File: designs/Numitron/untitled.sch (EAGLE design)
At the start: 10 parts, among them IC2 TLC5916IN, IC3 TLC5916IN, IC4 TLC5916IN, IC5 TLC5916IN

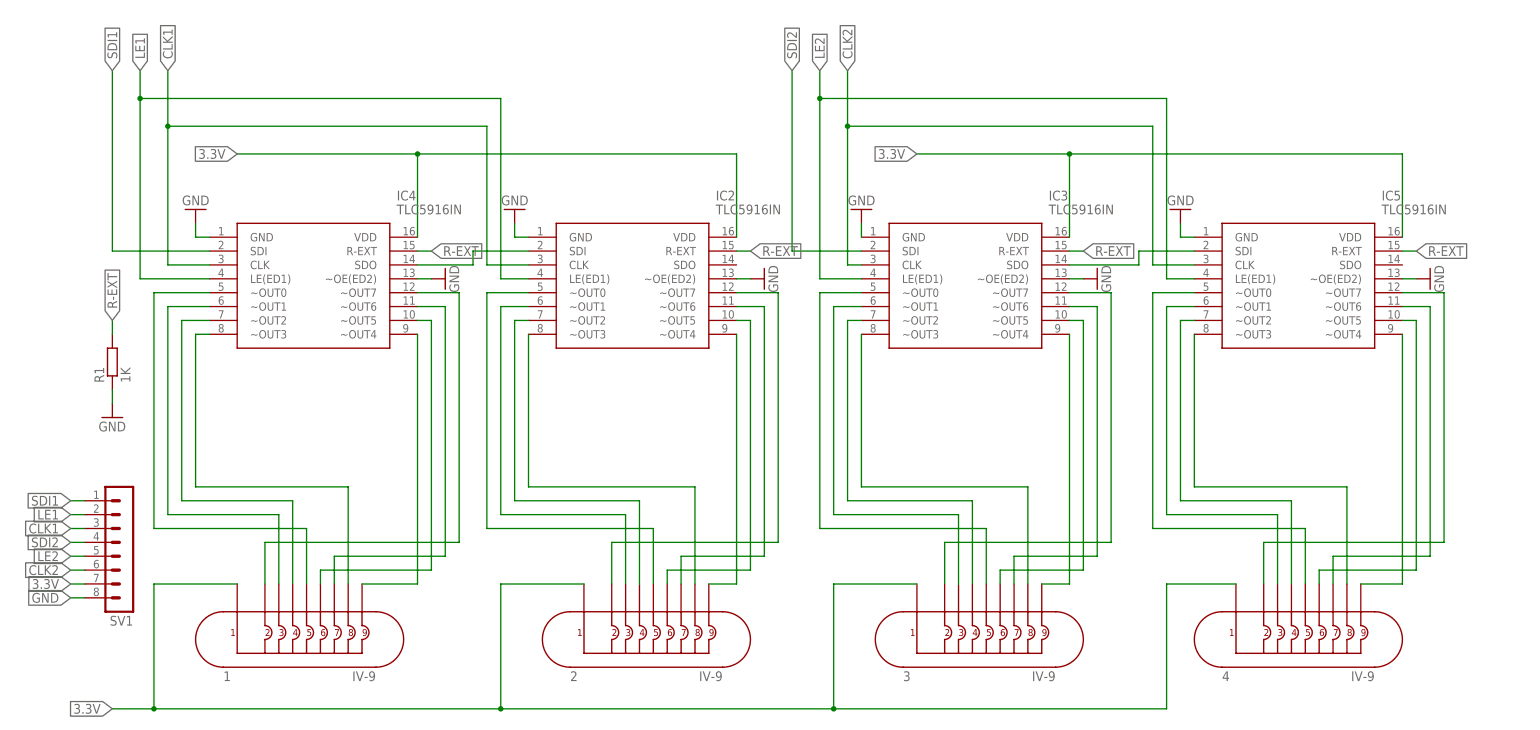
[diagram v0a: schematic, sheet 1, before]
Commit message: added designs Numitron modular first finish review tomorrow or tuesday
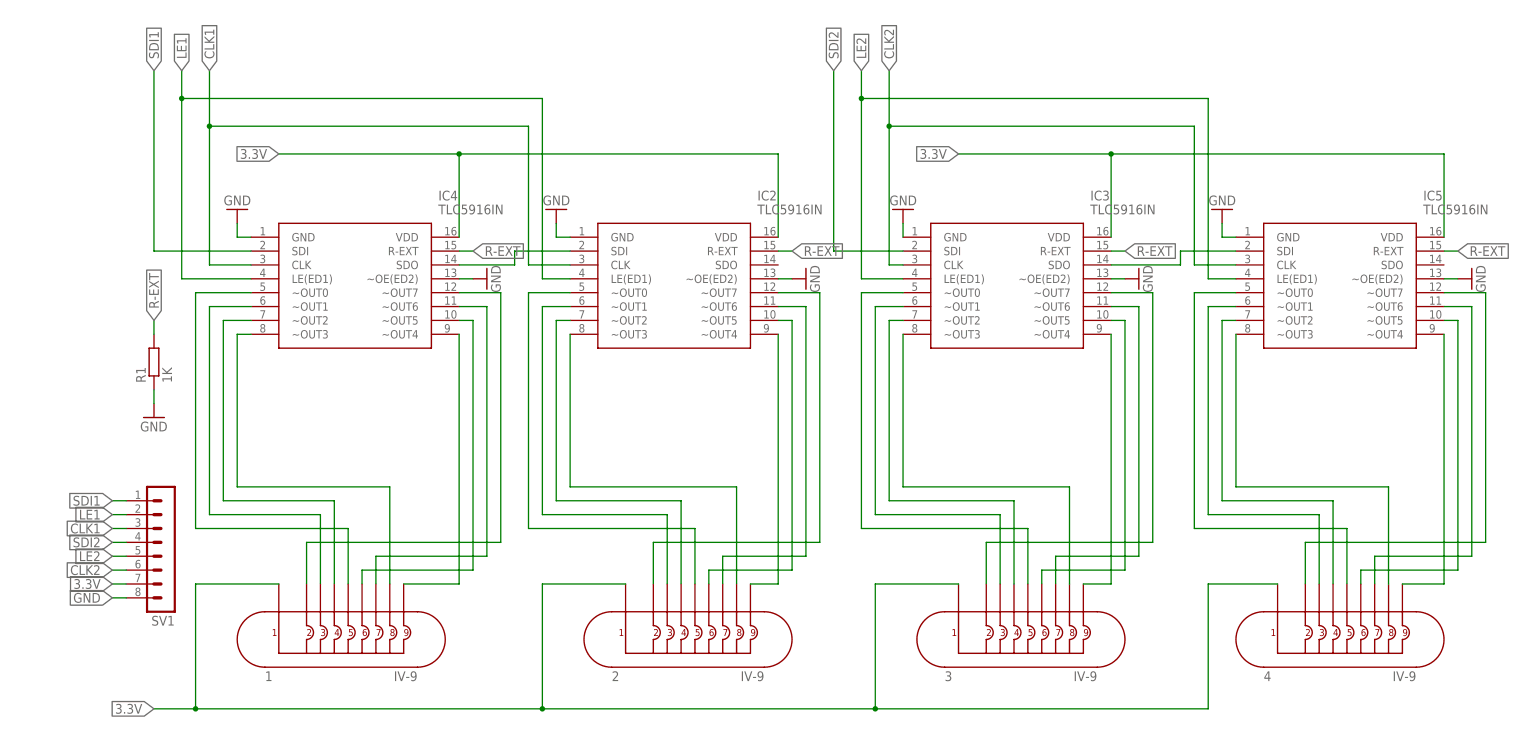
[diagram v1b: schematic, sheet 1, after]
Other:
- moved on the sheet: 1, 2, 3, 4, IC2, IC3, IC4, IC5, R1, SV1
